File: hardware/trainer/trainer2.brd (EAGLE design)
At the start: 82.1 x 54.3 mm, 63 parts, among them Q1 2N3906, Q2 2N3906, Q3 2N3906, Q4 2N3906

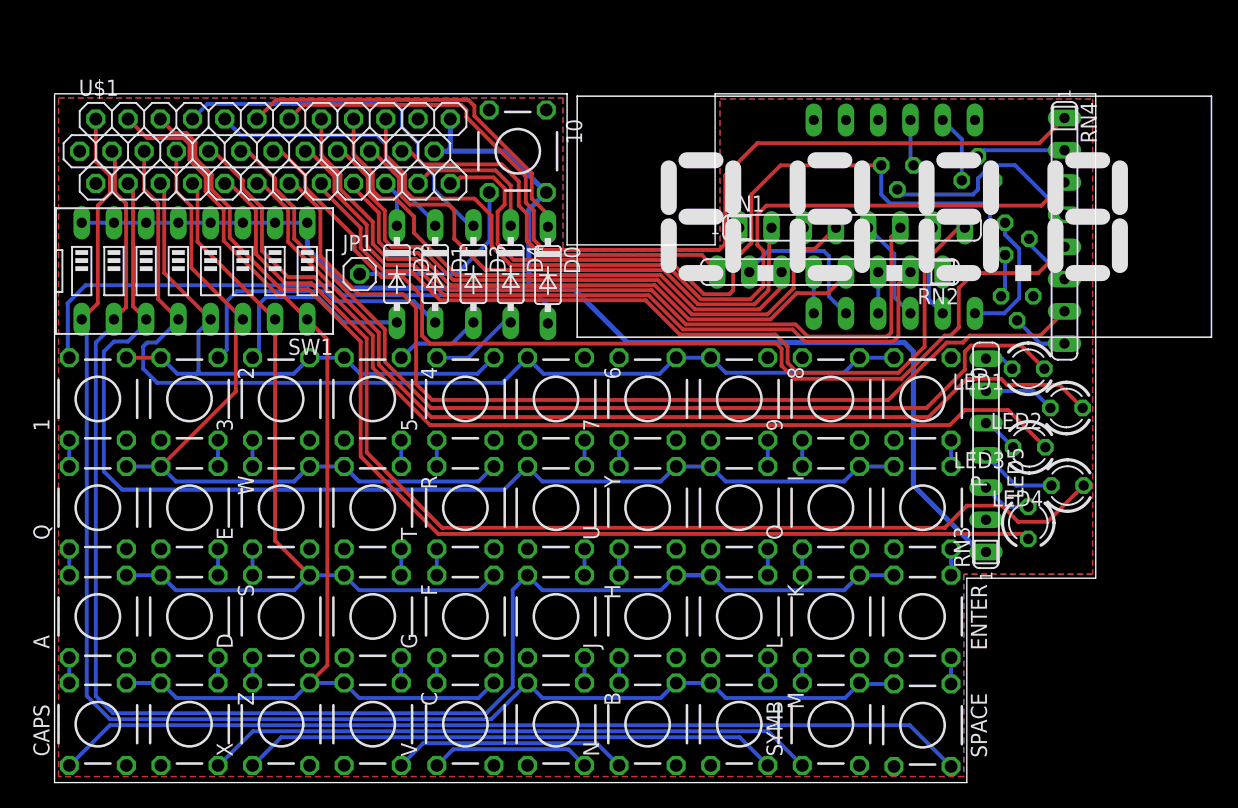
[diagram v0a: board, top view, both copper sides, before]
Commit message: Acabo trainer2
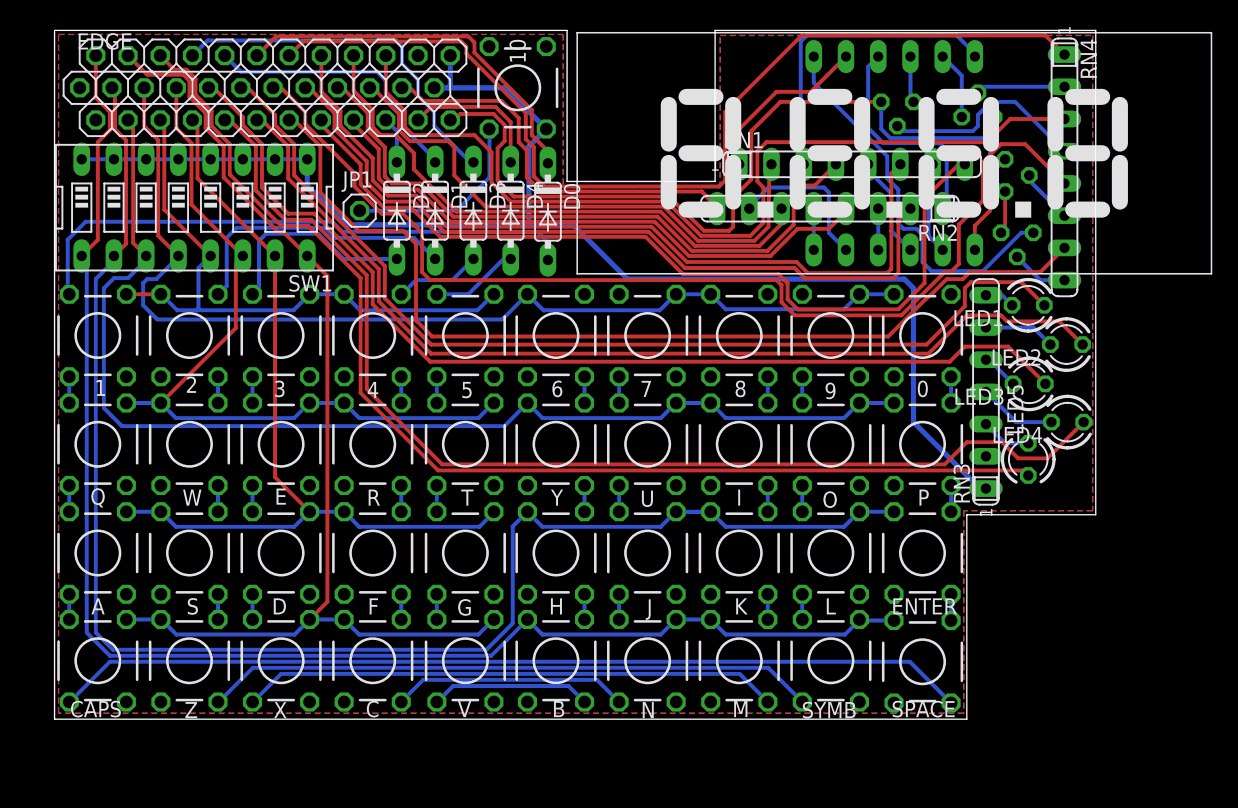
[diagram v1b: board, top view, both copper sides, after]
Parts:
- removed U$1: ZXUNO_CONNECTOR, zxuno:ZXUNO_CONNECTOR
- added EDGE: ZXUNO_CONNECTOR, zxuno:ZXUNO_CONNECTOR
- moved LED1 5.00 mm to (76.8, 32.6)
- moved LED3 5.00 mm to (76.8, 26.4)
- moved A 5.00 mm to (3.41, 13.1)
- moved D 5.00 mm to (17.9, 13.1)
- moved ENTER 5.00 mm to (68.4, 13.1)
- moved F 5.00 mm to (25.1, 13.1)
- moved G 5.00 mm to (32.4, 13.1)
- moved H 5.00 mm to (39.5, 13.1)
- moved J 5.00 mm to (46.8, 13.1)
- moved K 5.00 mm to (54.0, 13.1)
- moved L 5.00 mm to (61.2, 13.1)
- moved LED5 5.00 mm to (76.8, 20.5)
- moved S 5.00 mm to (10.6, 13.1)
- moved SPACE 5.00 mm to (68.4, 4.52)
- moved 0 5.00 mm to (68.4, 30.2)
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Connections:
- net 3.3V: now also EDGE.3.3V@1; no longer U$1.3.3V@1
- net 5V: now also EDGE.5V; no longer U$1.5V
- net A10: now also EDGE.P14; no longer U$1.P14
- net A11: now also EDGE.P10; no longer U$1.P10
- net A12: now also EDGE.P11; no longer U$1.P11
- net A13: now also EDGE.P7; no longer U$1.P7
- net A14: now also EDGE.P8; no longer U$1.P8
- net A15: now also EDGE.P6; no longer U$1.P6
- net A8: now also EDGE.P9; no longer U$1.P9
- net A9: now also EDGE.P13; no longer U$1.P13
- net COL0: now also EDGE.P21; no longer U$1.P21
- net COL1: now also EDGE.P18; no longer U$1.P18
- net COL2: now also EDGE.P31; no longer U$1.P31
- net COL3: now also EDGE.P15; no longer U$1.P15
- net COL4: now also EDGE.P34; no longer U$1.P34
- net DIG1: now also EDGE.P22; no longer U$1.P22
- net DIG2: now also EDGE.P33; no longer U$1.P33
- net DIG3: now also EDGE.P24; no longer U$1.P24
- net DIG4: now also EDGE.P23; no longer U$1.P23
- net DISA: now also EDGE.P32; no longer U$1.P32
- net DISB: now also EDGE.P29; no longer U$1.P29
- net DISC: now also EDGE.P27; no longer U$1.P27
- net DISD: now also EDGE.P25; no longer U$1.P25
- net DISDP: now also EDGE.P35; no longer U$1.P35
- net DISE: now also EDGE.P26; no longer U$1.P26
- net DISF: now also EDGE.P28; no longer U$1.P28
- net DISG: now also EDGE.P30; no longer U$1.P30
- net GND: now also EDGE.GND@1, EDGE.GND@2; no longer U$1.GND@1, U$1.GND@2
- net LED1: now also EDGE.P20; no longer U$1.P20
- net LED2: now also EDGE.P19; no longer U$1.P19
- net LED3: now also EDGE.P17; no longer U$1.P17
- net LED4: now also EDGE.P16; no longer U$1.P16
- net LED5: now also EDGE.P12; no longer U$1.P12
- net VCC: now also EDGE.3.3V@2; no longer U$1.3.3V@2
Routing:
- net N$4: track 0.00 -> 30.6 mm
- net N$10: track 0.00 -> 24.5 mm
- net N$14: track 0.00 -> 17.6 mm
- net N$9: track 0.00 -> 13.6 mm
- net DIG4: track 79.7 -> 84.0 mm
- net N$1: track 10.4 -> 8.13 mm
- net DIG3: track 76.7 -> 77.9 mm
